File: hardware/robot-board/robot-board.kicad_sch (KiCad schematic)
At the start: 74 parts, among them J1 USB_C_Receptacle_USB2.0_14P, J2 Conn_01x03_Pin, J3 Conn_01x03_Pin, J4 Conn_01x03_Pin, J5 Conn_01x03_Pin, Q1 BSS138, Q2 BSS138, Q3 BSS138, Q4 BSS138, SW1 SW_SPST, U1 ESP32-S3-WROOM-1, U2 LMR51450, U3 LMR51450, U4 TPS61088, U6 TVS0500DRV

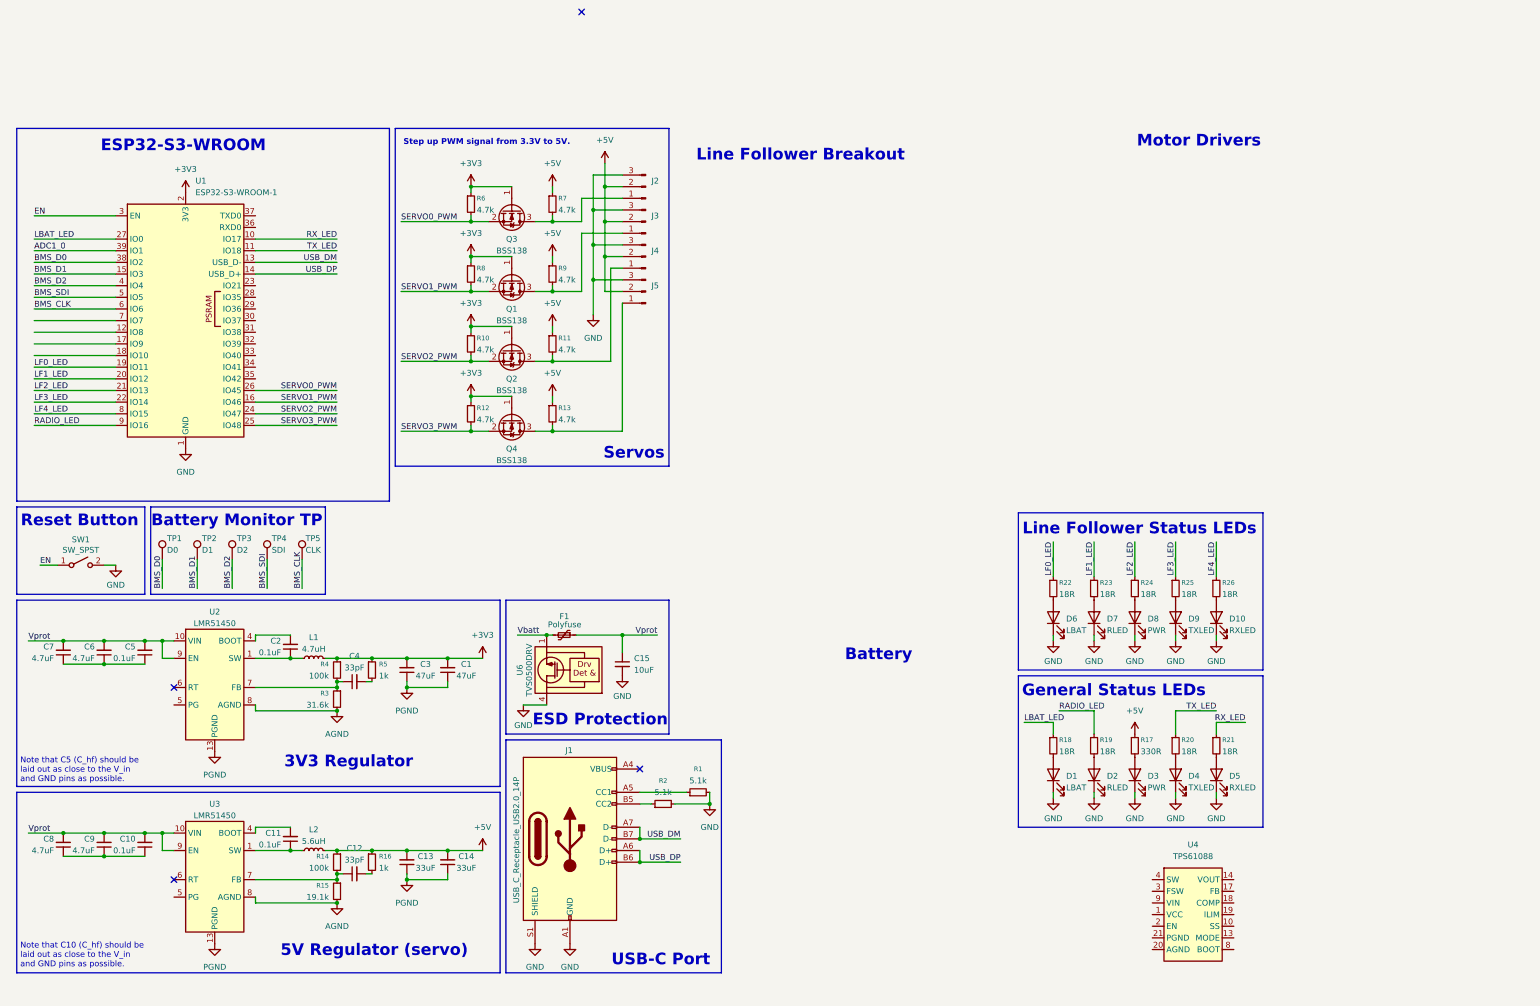
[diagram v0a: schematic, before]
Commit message: finished most of schematic
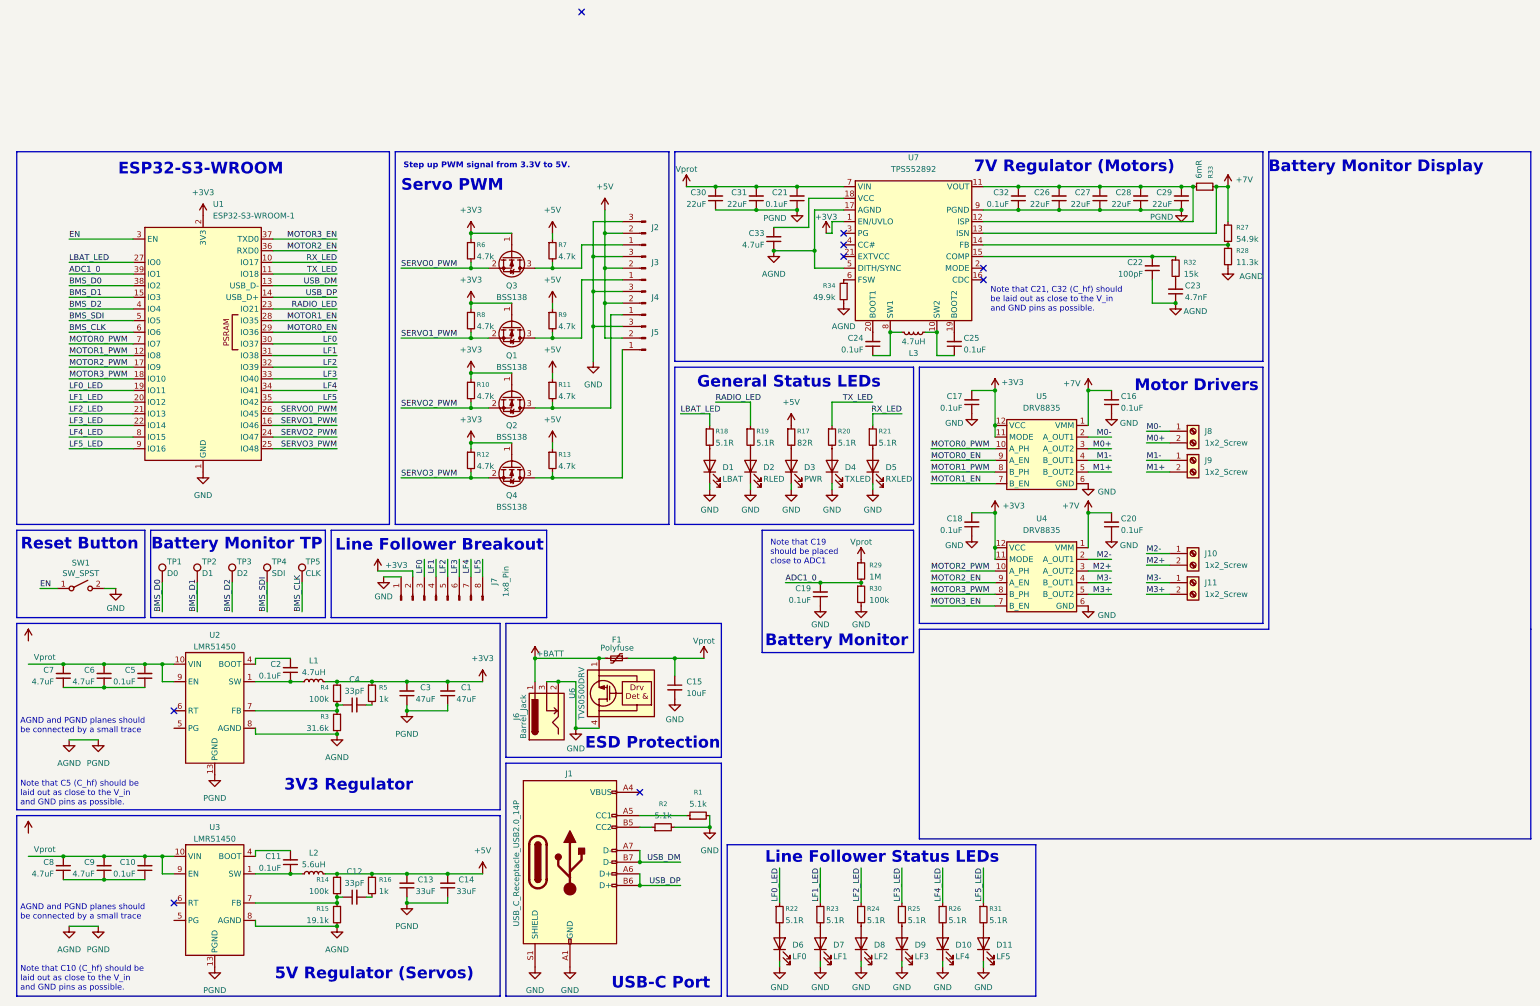
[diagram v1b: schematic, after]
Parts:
- removed U4: TPS61088, Package_DFN_QFN:Texas_VQFN-RHL-20_ThermalVias, symbol Regulator_Switching:TPS61088
- added C16, C17, C18, C19, C20, C21, C24, C25, C32: 0.1uF, Capacitor_SMD:C_0402_1005Metric, symbol Device:C_Small
- added C22: 100pF, Capacitor_SMD:C_0402_1005Metric, symbol Device:C_Small
- added C23: 4.7nF, Capacitor_SMD:C_0402_1005Metric, symbol Device:C_Small
- added C26, C27, C28, C29, C30, C31: 22uF, Capacitor_SMD:C_0402_1005Metric, symbol Device:C_Small
- added C33: 4.7uF, Capacitor_SMD:C_0402_1005Metric, symbol Device:C_Small
- added D11: LF5, LED_SMD:LED_1206_3216Metric, symbol Device:LED
- added J10, J11, J8, J9: 1x2_Screw, RedRobotFootprints:ScrewTerminalP3.5mm, symbol Connector:Screw_Terminal_01x02
- added J6: Barrel_Jack, Connector_BarrelJack:BarrelJack_Horizontal, symbol Connector:Barrel_Jack_Switch
- added J7: 1x8_Pin, Connector_PinHeader_2.54mm:PinHeader_1x08_P2.54mm_Vertical_SMD_Pin1Left, symbol Connector:Conn_01x08_Pin
- added L3: 4.7uH, Inductor_SMD:L_Bourns_SRP7028A_7.3x6.6mm, symbol Device:L_Small
- added R27: 54.9k, Resistor_SMD:R_0603_1608Metric, symbol Device:R_Small
- added R28: 11.3k, Resistor_SMD:R_0603_1608Metric, symbol Device:R_Small
- added R29: 1M, Resistor_SMD:R_0603_1608Metric, symbol Device:R_Small
- added R30: 100k, Resistor_SMD:R_0603_1608Metric, symbol Device:R_Small
- added R31: 5.1R, Resistor_SMD:R_0402_1005Metric, symbol Device:R_Small
- added R32: 15k, Resistor_SMD:R_0603_1608Metric, symbol Device:R_Small
- added R33: 6mR, Resistor_SMD:R_0603_1608Metric, symbol Device:R_Small
- added R34: 49.9k, Resistor_SMD:R_0603_1608Metric, symbol Device:R_Small
- added U4, U5: DRV8835, Package_SON:WSON-12-1EP_3x2mm_P0.5mm_EP1x2.65, symbol Driver_Motor:DRV8835
- added U7: TPS552892, symbol Regulator_Switching:TPS552892
- C1, C10, C11, C12, C13, C14, C15, C2, C3, C4, C5, C6, C7, C8, C9: footprint (none) -> Capacitor_SMD:C_0402_1005Metric
- D1, D2, D3, D4, D5: footprint (none) -> LED_SMD:LED_1206_3216Metric
- D10: value RXLED -> LF4; footprint (none) -> LED_SMD:LED_1206_3216Metric
- D6: value LBAT -> LF0; footprint (none) -> LED_SMD:LED_1206_3216Metric
- D7: value RLED -> LF1; footprint (none) -> LED_SMD:LED_1206_3216Metric
- D8: value PWR -> LF2; footprint (none) -> LED_SMD:LED_1206_3216Metric
- D9: value TXLED -> LF3; footprint (none) -> LED_SMD:LED_1206_3216Metric
- J1: footprint (none) -> footprints:USB_C_Receptacle_GCT_USB4105-xx-A_16P_TopMnt_Horizontal
- J2, J3, J4, J5: footprint (none) -> Connector_PinHeader_2.54mm:PinHeader_1x02_P2.54mm_Vertical_SMD_Pin1Right
- L1, L2: footprint (none) -> Inductor_SMD:L_Bourns_SRP7028A_7.3x6.6mm
- R1, R10, R11, R12, R13, R2, R6, R7, R8, R9: footprint (none) -> Resistor_SMD:R_0402_1005Metric
- R14, R15, R16, R3, R4, R5: footprint (none) -> Resistor_SMD:R_0603_1608Metric
- R17: value 330R -> 82R; footprint (none) -> Resistor_SMD:R_0402_1005Metric
- R18, R19, R20, R21, R22, R23, R24, R25, R26: value 18R -> 5.1R; footprint (none) -> Resistor_SMD:R_0402_1005Metric
- SW1: footprint (none) -> random-keyboard-parts:SKQGADE010
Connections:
- net PGND is gone; now on net AGND: C1.1, C13.1, C14.1, C3.1, U2.13 (PGND), U3.13 (PGND)
- net +3V3: now also C17.2, C18.2, J7.2 (Pin_2), U4.11 (MODE), U4.12 (VCC), U5.11 (MODE), U5.12 (VCC), U7.1 (EN/UVLO)
- net ADC1_0: now also C19.2, R29.2, R30.1
- net AGND: now also C21.1, C22.1, C23.1, C26.1, C27.1, C28.1, C29.1, C30.1, C31.1, C32.1, C33.1, R28.2, R34.2, U7.17 (AGND), U7.5 (DITH/SYNC), U7.9 (PGND)
- net GND: now also C16.1, C17.1, C18.1, C19.1, C20.1, D11.1 (K), J6.2, J6.3, J7.1 (Pin_1), R30.2, U4.6 (GND), U5.6 (GND)
- net RADIO_LED: now also U1.23 (IO21); no longer U1.9 (IO16)
- net VIN: no longer C15.1, F1.1
- net MOTOR1_PWM: now reaches U1.12 (IO8)
- net MOTOR1_PWM: now also U5.8 (B_PH)
- net MOTOR2_PWM: now reaches U1.17 (IO9)
- net MOTOR2_PWM: now also U4.10 (A_PH)
- net MOTOR3_PWM: now reaches U1.18 (IO10)
- net MOTOR3_PWM: now also U4.8 (B_PH)
- net MOTOR1_EN: now reaches U1.28 (IO35)
- net MOTOR1_EN: now also U5.7 (B_EN)
- net MOTOR0_EN: now reaches U1.29 (IO36)
- net MOTOR0_EN: now also U5.9 (A_EN)
- net LF0: now reaches U1.30 (IO37)
- net LF0: now also J7.3 (Pin_3)
- net LF1: now reaches U1.31 (IO38)
- net LF1: now also J7.4 (Pin_4)
- net LF2: now reaches U1.32 (IO39)
- net LF2: now also J7.5 (Pin_5)
- net LF3: now reaches U1.33 (IO40)
- net LF3: now also J7.6 (Pin_6)
- net LF4: now reaches U1.34 (IO41)
- net LF4: now also J7.7 (Pin_7)
- net LF5: now reaches U1.35 (IO42)
- net LF5: now also J7.8 (Pin_8)
- net MOTOR2_EN: now reaches U1.36 (RXD0)
- net MOTOR2_EN: now also U4.9 (A_EN)
- net MOTOR3_EN: now reaches U1.37 (TXD0)
- net MOTOR3_EN: now also U4.7 (B_EN)
- net MOTOR0_PWM: now reaches U1.7 (IO7)
- net MOTOR0_PWM: now also U5.10 (A_PH)
- net Vbatt renamed +BATT
- net +BATT: now also J6.1
- new net: R34.1, U7.6 (FSW)
- new net: C25.1, L3.1, U7.10 (SW2)
- new net: C24.1, L3.2, U7.8 (SW1)
- new net: C22.2, R32.1, U7.15 (COMP)
- new net: R27.2, R28.1, U7.14 (FB)
- new net: C26.2, C27.2, C28.2, C29.2, C32.2, R33.2, U7.11 (VOUT), U7.12 (ISP)
- new net: C24.2, U7.20 (BOOT1)
- new net: C33.2, U7.18 (VCC)
- new net: C25.2, U7.19 (BOOT2)
- new net: C23.2, R32.2
- new net: D11.2 (A), R31.2
- new net +7V: C16.2, C20.2, R27.1, R33.1, U4.1 (VMM), U5.1 (VMM), U7.13 (ISN)
- new net LF5_LED: R31.1, U1.9 (IO16)
- new net M0+: J8.2 (Pin_2), U5.3 (A_OUT2)
- new net M0-: J8.1 (Pin_1), U5.2 (A_OUT1)
- new net M1+: J9.2 (Pin_2), U5.5 (B_OUT2)
- new net M1-: J9.1 (Pin_1), U5.4 (B_OUT1)
- new net M2+: J10.2 (Pin_2), U4.3 (A_OUT2)
- new net M2-: J10.1 (Pin_1), U4.2 (A_OUT1)
- new net M3+: J11.2 (Pin_2), U4.5 (B_OUT2)
- new net M3-: J11.1 (Pin_1), U4.4 (B_OUT1)
- new net Vprot: C15.1, C21.2, C30.2, C31.2, F1.1, R29.1, U7.7 (VIN)
- no-connect marks 4 -> 9
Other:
- note added: "5V Regulator (Servos)"
- note added: "7V Regulator (Motors)"
- note added: "AGND and PGND planes should be connected by a small trace"
- note added: "Battery Monitor"
- note added: "Battery Monitor Display"
- note added: "Note that C19 should be placed close to ADC1"
- note added: "Note that C21, C32 (C_hf) should be laid out as close to the V_in and GND pins as possible."
- note added: "Servo PWM"
- note removed: "5V Regulator (servo)"
- note removed: "Battery"
- note removed: "Servos"
- moved on the sheet: C1, C10, C11, C12, C13, C14, C15, C2, C3, C4, C5, C6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
